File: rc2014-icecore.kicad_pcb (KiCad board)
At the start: 2 copper layers, 100.1 x 63.3 mm, 18 parts, among them J1 Conn_02x40_Top_Bottom, J3 Conn_02x15_Odd_Even, J5 Conn_02x13_Odd_Even, U1 SN74CB3T3245, U2 SN74CB3T3245, U3 SN74CB3T3245, U4 SN74CB3T3245, U5 SN74CB3T3245, U6 LM1117-3.3

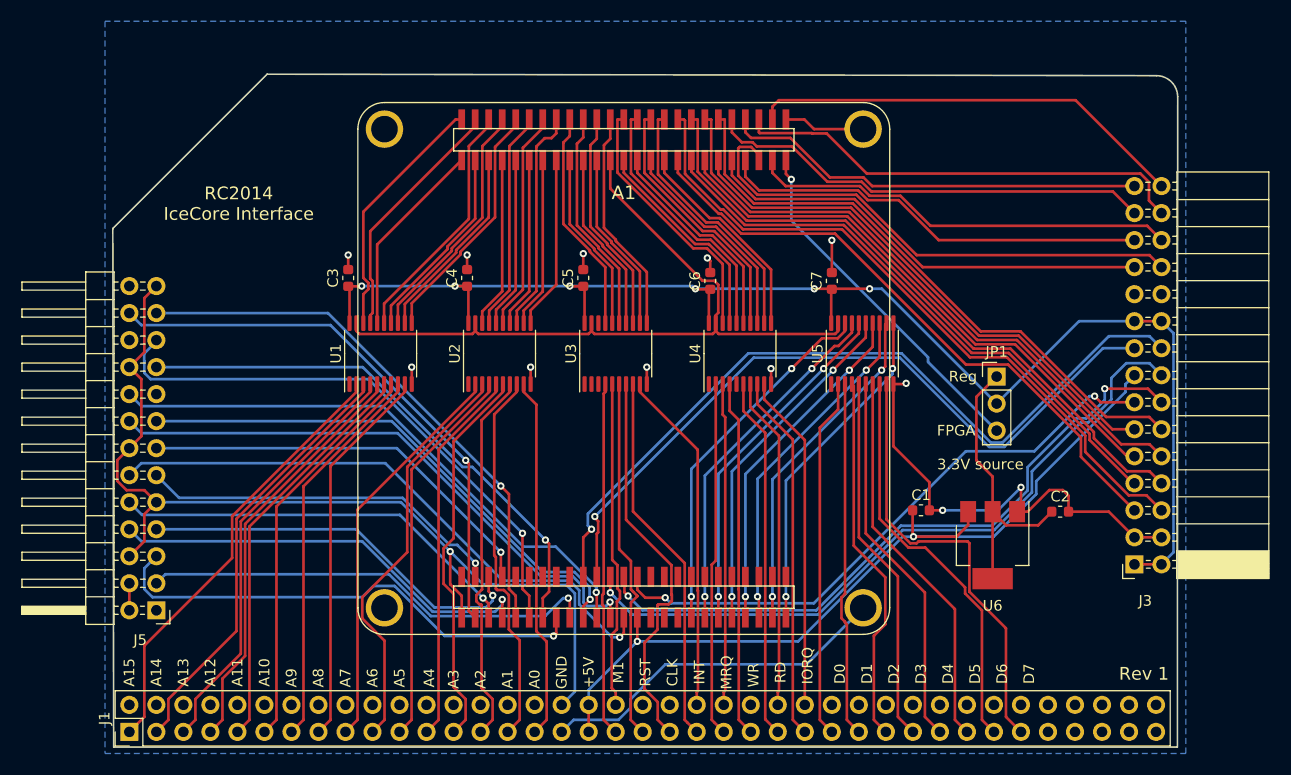
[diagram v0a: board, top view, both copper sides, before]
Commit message: Board redesign
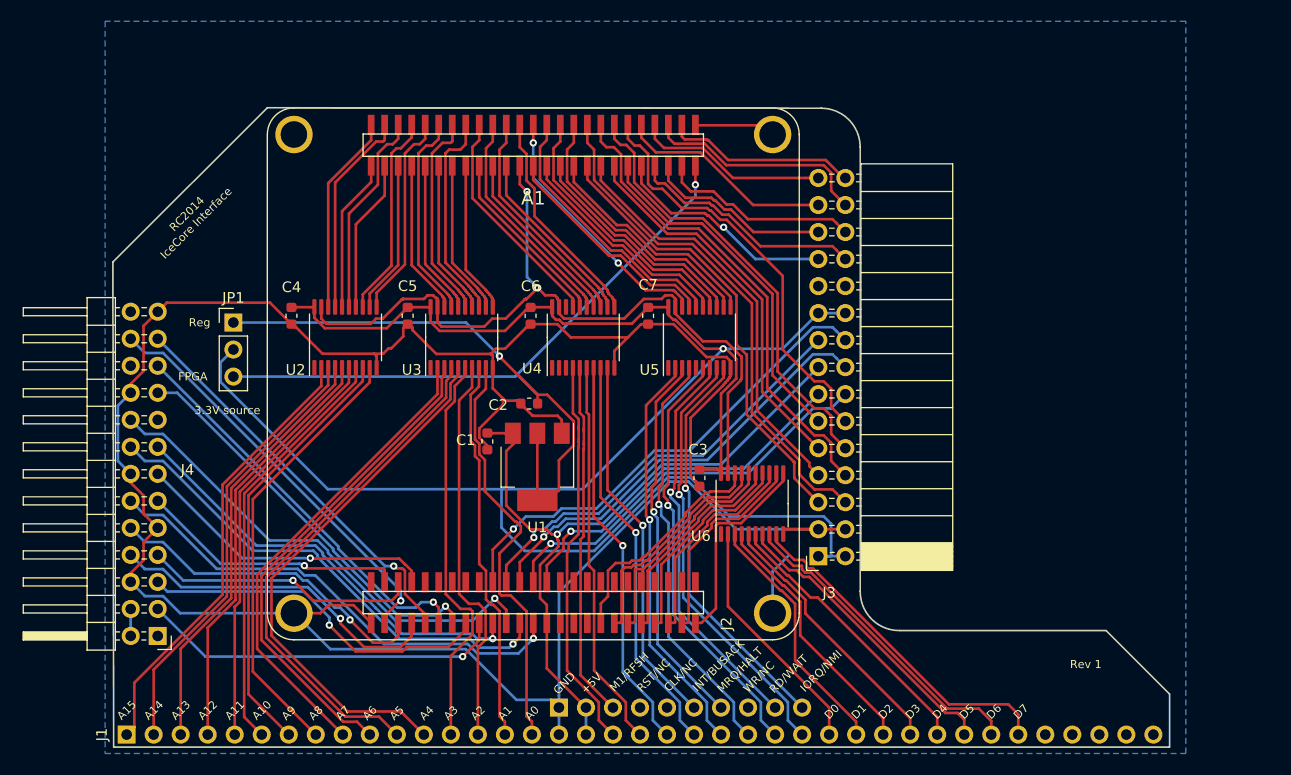
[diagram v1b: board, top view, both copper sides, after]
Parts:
- added J2: Conn_01x10, rc2014:PinHeader_1x10_P2.54mm_Vertical_NoSilk, F.Cu at (102.4, 160.8)
- J1: value Conn_02x40_Top_Bottom -> Conn_01x39; footprint Connector_PinHeader_2.54mm:PinHeader_2x39_P2.54mm_Vertical -> rc2014:PinHeader_1x39_P2.54mm_Vertical_NoSilk
- moved JP1 71.9 mm to (71.8, 124.6)
- moved C2 50.9 mm to (99.6, 132.2), turned to 180 degrees
- moved U1 43.4 mm to (100.3, 138.2)
- moved C1 41.3 mm to (95.6, 135.8), turned to 270 degrees
- moved J3 29.7 mm to (126.7, 146.6)
- moved C3 22.3 mm to (115.6, 139.2), turned to 270 degrees
- moved U6 17.5 mm to (120.5, 141.6)
- moved A1 8.52 mm to (84.7, 105.9)
- moved C7 6.70 mm to (110.7, 124.0), turned to 270 degrees
- moved C5 6.62 mm to (88.1, 124.0), turned to 270 degrees
- moved C4 6.41 mm to (77.2, 124.0), turned to 270 degrees
- moved C6 6.10 mm to (99.7, 124.0), turned to 270 degrees
- moved U5 4.10 mm to (115.6, 126.0)
- moved U3 3.87 mm to (93.2, 126.0)
- moved U2 3.64 mm to (82.3, 126.0)
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- renumbered C7 to C3, C3 to C4, C4 to C5, C5 to C6, C6 to C7, J5 to J4, U6 to U1, U1 to U2, U2 to U3, U3 to U4, U4 to U5, U5 to U6
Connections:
- J1 pad 10: (no net) -> /A6
- J1 pad 11: /A10 -> /A5
- J1 pad 12: (no net) -> /A4
- J1 pad 13: /A9 -> /A3
- J1 pad 14: (no net) -> /A2
- J1 pad 15: /A8 -> /A1
- J1 pad 16: (no net) -> /A0
- J1 pad 17: /A7 -> GND
- J1 pad 18: (no net) -> +5V
- J1 pad 19: /A6 -> /M1
- J1 pad 2: (no net) -> /A14
- J1 pad 20: (no net) -> //RESET
- J1 pad 21: /A5 -> /CLK
- J1 pad 22: (no net) -> /INT
- J1 pad 23: /A4 -> /MREQ
- J1 pad 24: (no net) -> //WR
- J1 pad 25: /A3 -> //RD
- J1 pad 26: (no net) -> //IORQ
- J1 pad 27: /A2 -> /D0
- J1 pad 28: (no net) -> /D1
- J1 pad 29: /A1 -> /D2
- J1 pad 3: /A14 -> /A13
- J1 pad 30: (no net) -> /D3
- J1 pad 31: /A0 -> /D4
- J1 pad 32: (no net) -> /D5
- J1 pad 33: GND -> /D6
- J1 pad 34: GND -> /D7
- J1 pad 35: +5V -> (no net)
- J1 pad 36: +5V -> (no net)
- J1 pad 37: /M1 -> (no net)
- J1 pad 38: /~RFSH -> (no net)
- J1 pad 39: //RESET -> (no net)
- J1 pad 4: (no net) -> /A12
- J1 pad 5: /A13 -> /A11
- J1 pad 6: (no net) -> /A10
- J1 pad 7: /A12 -> /A9
- J1 pad 8: (no net) -> /A8
- J1 pad 9: /A11 -> /A7
- J3 pad 24: /P46 -> /P43
- J3 pad 25: /P43 -> /P46
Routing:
- net GND: track 191.8 -> 246.3 mm, vias 13 -> 0
- net +3V3: track 131.5 -> 184.7 mm, vias 6 -> 1
- net /P46: track 48.7 -> 17.5 mm
- net /AN6: track 70.1 -> 40.0 mm
- net /AN5: track 74.7 -> 45.4 mm
- net Net-(C2-Pad1): track 27.0 -> 55.2 mm, vias 0 -> 1
- net /AN8: track 63.7 -> 37.8 mm, vias 2 -> 1
- net /AN7: track 66.7 -> 41.2 mm
- net /P45: track 41.4 -> 18.1 mm
- net /AN9: track 56.8 -> 34.3 mm, vias 2 -> 1
- net /P44: track 43.2 -> 21.5 mm
- net /P40: track 42.2 -> 20.5 mm
- net /P41: track 39.9 -> 18.2 mm
- net /P42: track 42.9 -> 21.3 mm, vias 0 -> 1
- net /P47: track 40.4 -> 18.9 mm
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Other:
- board size 100.1 x 63.3 mm -> 99.3 x 60.1 mm
- board text added: "CLK/NC"
- board text added: "INT/BUSACK"
- board text added: "IORQ/NMI"
- board text added: "M1/RFSH"
- board text added: "MRQ/HALT"
- board text added: "RD/WAIT"
- board text added: "RST/NC"
- board text added: "WR/NC"
- board text removed: "CLK"
- board text removed: "INT"
- board text removed: "IORQ"
- board text removed: "M1"
- board text removed: "MRQ"
- board text removed: "RD"
- board text removed: "RST"
- board text removed: "WR"
